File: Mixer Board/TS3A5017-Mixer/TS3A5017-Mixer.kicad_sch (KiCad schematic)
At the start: 10 parts, among them J1 RF-In, J2 CLK0, J3 CLK1, J4 Conn_01x06, U1 TS3A5017RGY

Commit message: Finish first iteration, generate manufacturing files
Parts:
- J1, J2, J3: footprint Connector_Coaxial:SMA_Amphenol_901-143_Horizontal -> Connector_Amphenol:AMPHENOL_901-143-6RFX
- J4: footprint (none) -> Connector_PinHeader_2.54mm:PinHeader_1x06_P2.54mm_Vertical
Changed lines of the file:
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@@
 			)
 		)
-		(property "Footprint" ""
+		(property "Footprint" "Connector_PinHeader_2.54mm:PinHeader_1x06_P2.54mm_Vertical"
 			(at 189.23 97.79 0)
 			(effects
@@
 			)
 		)
-		(property "Footprint" "Connector_Coaxial:SMA_Amphenol_901-143_Horizontal"
+		(property "Footprint" "Connector_Amphenol:AMPHENOL_901-143-6RFX"
 			(at 85.09 96.52 0)
 			(effects
@@
 			)
 		)
-		(property "Footprint" "Connector_Coaxial:SMA_Amphenol_901-143_Horizontal"
+		(property "Footprint" "Connector_Amphenol:AMPHENOL_901-143-6RFX"
 			(at 85.09 106.68 0)
 			(effects
@@
 			)
 		)
-		(property "Footprint" "Connector_Coaxial:SMA_Amphenol_901-143_Horizontal"
+		(property "Footprint" "Connector_Amphenol:AMPHENOL_901-143-6RFX"
 			(at 85.09 116.84 0)
 			(effects

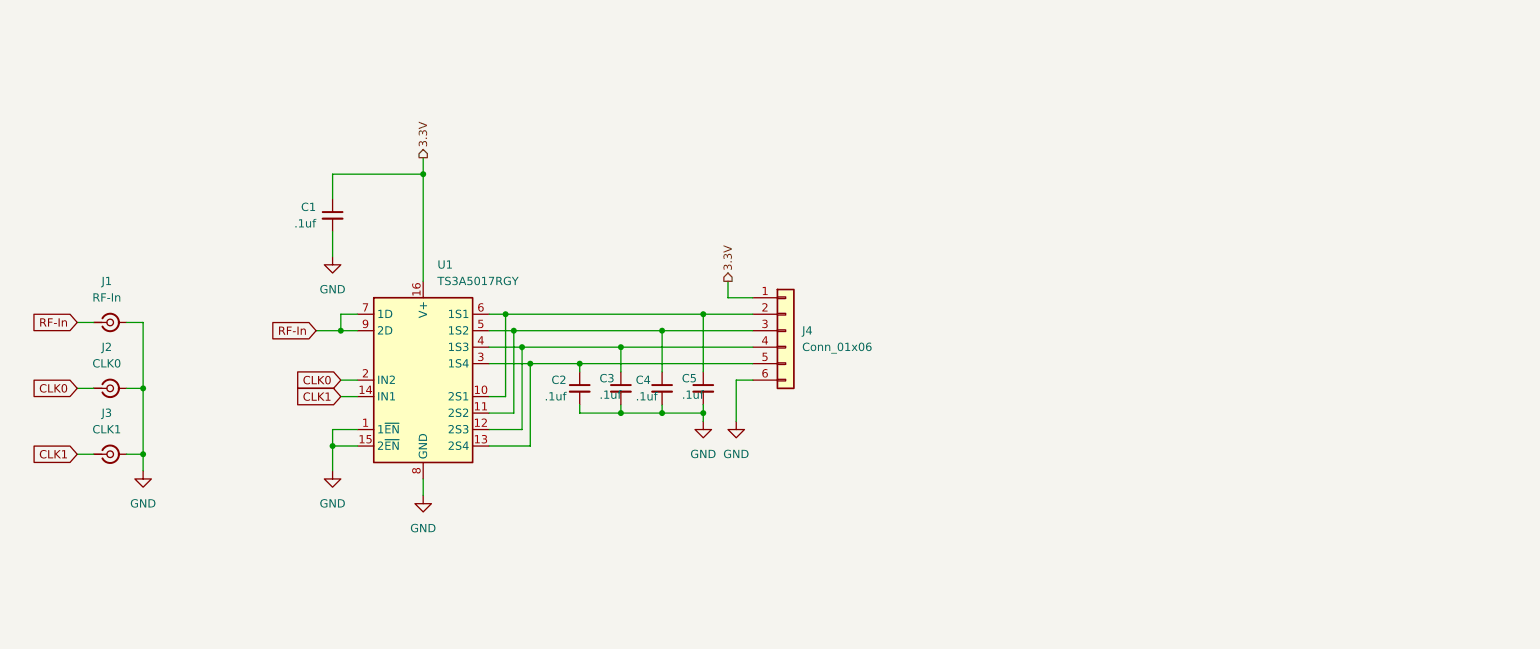
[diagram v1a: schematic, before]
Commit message: Working on mixer board
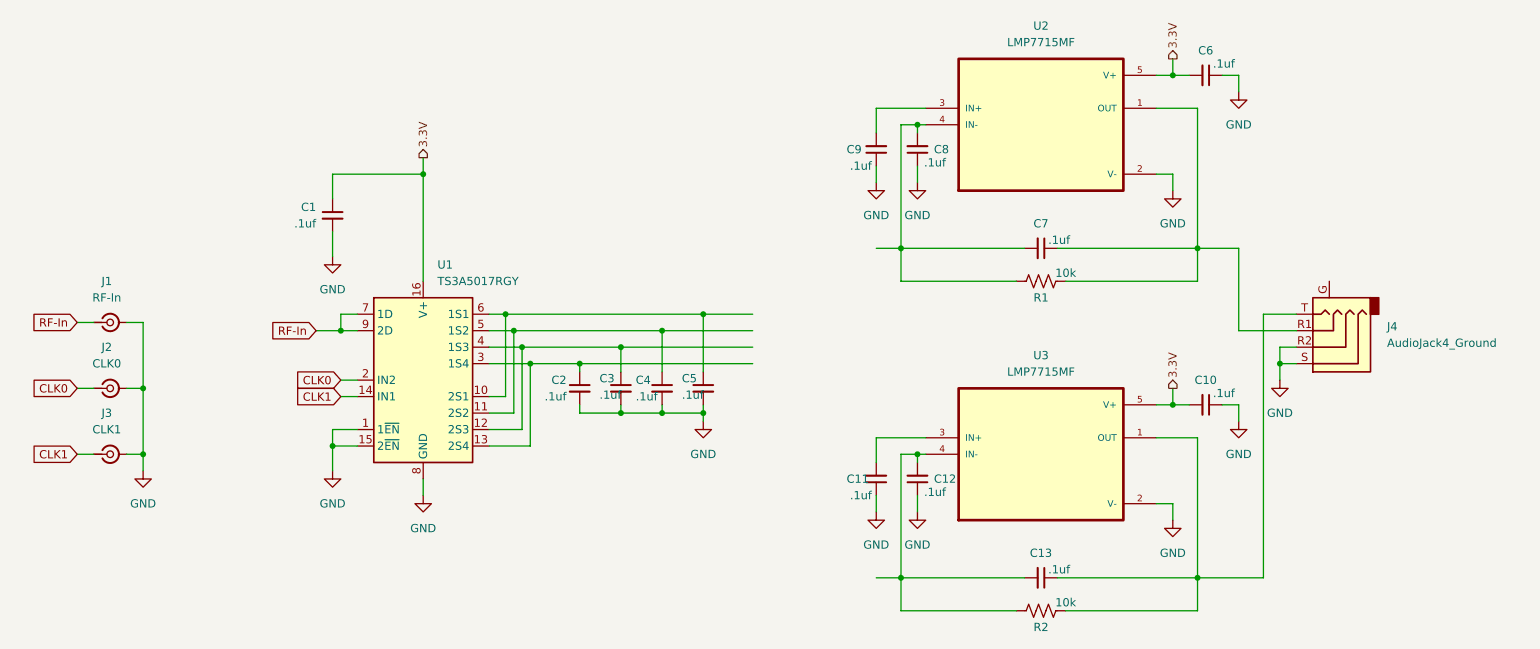
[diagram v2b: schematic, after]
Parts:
- removed J4: Conn_01x06, Connector_PinHeader_2.54mm:PinHeader_1x06_P2.54mm_Vertical, symbol Connector_Generic:Conn_01x06
- added C10, C11, C12, C13, C6, C7, C8, C9: .1uf, Capacitor_SMD:C_0201_0603Metric, symbol Device:C_Small
- added J4: AudioJack4_Ground, Connector_Audio:Jack_3.5mm_CUI_SJ-3523-SMT_Horizontal, symbol Connector_Audio:AudioJack4_Ground
- added R1, R2: 10k, Resistor_SMD:R_0201_0603Metric, symbol Device:R_US
- added U2, U3: LMP7715MF, Package_TO_SOT_SMD:SOT-23-5, symbol Amplifier_Operational:LMP7715MF
- J1, J2, J3: footprint Connector_Amphenol:AMPHENOL_901-143-6RFX -> Connector_Coaxial:SMA_Amphenol_901-143_Horizontal
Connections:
- net 3.3V: now also C10.2, C6.2, U2.5 (V+), U3.5 (V+)
- net GND: now also C10.1, C11.1, C12.1, C6.1, C8.1, C9.1, J4.R2, J4.S, U2.2 (V-), U3.2 (V-)
- new net: C12.2, C13.2, R2.1, U3.4 (IN-)
- new net: C7.1, J4.R1, R1.2, U2.1 (OUT)
- new net: C13.1, J4.T, R2.2, U3.1 (OUT)
- new net: C7.2, C8.2, R1.1, U2.4 (IN-)
- new net: C9.2, U2.3 (IN+)
- new net: C11.2, U3.3 (IN+)
